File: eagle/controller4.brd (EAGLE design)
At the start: 117.8 x 48.2 mm, 30 parts, among them K1 SRD-05VDC-SL-C, K2 SRD-05VDC-SL-C, K3 SRD-05VDC-SL-C, K4 SRD-05VDC-SL-C, T1 BC547, T2 BC547, T3 BC547, T4 BC547, X1 VCC, X2 IN1, X3 IN2, X4 IN3, X5 IN4

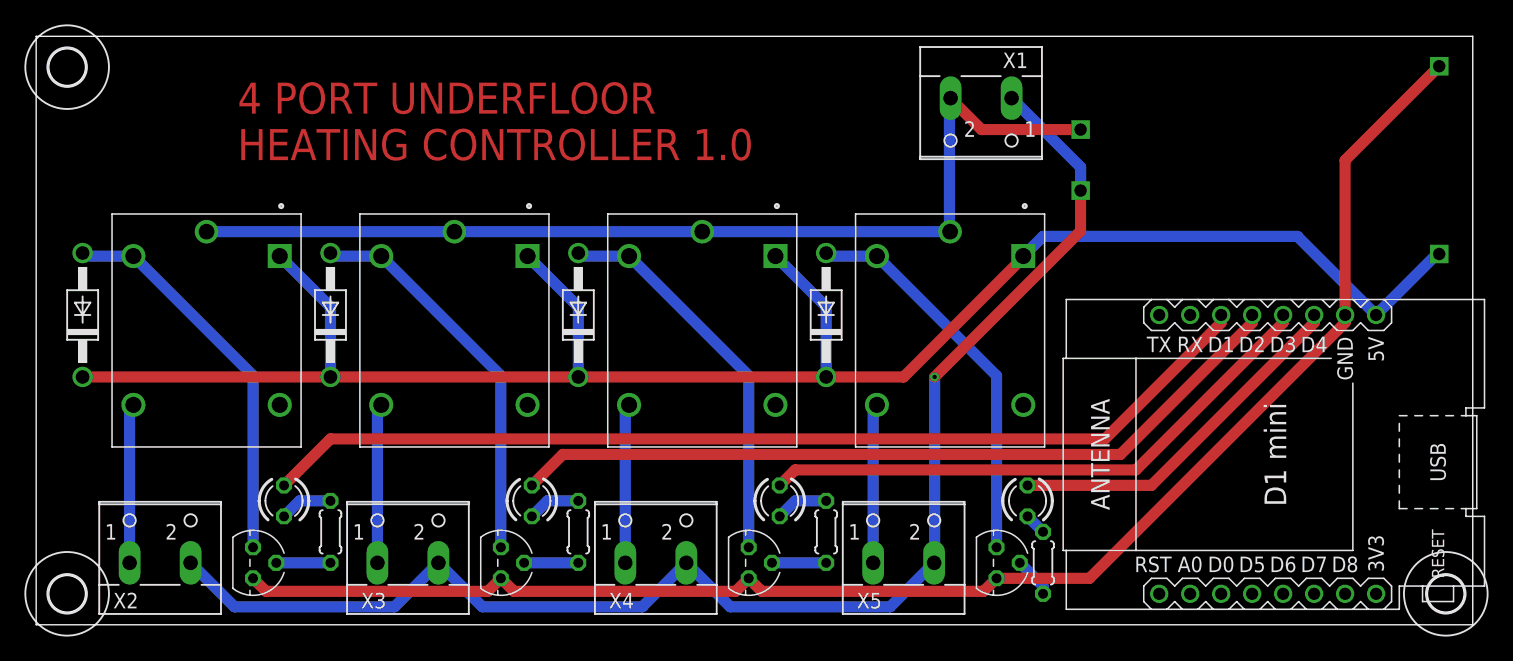
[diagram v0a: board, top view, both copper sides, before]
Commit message: Update to Version 1.1
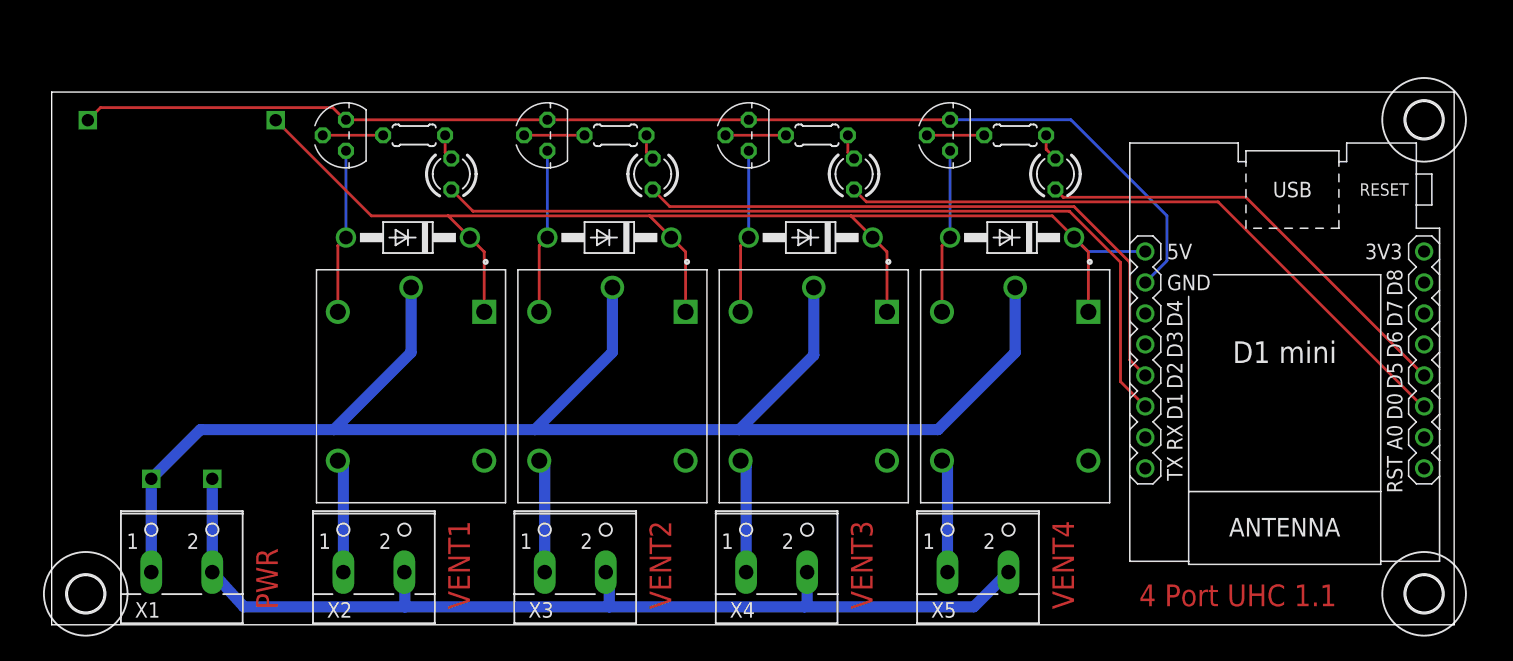
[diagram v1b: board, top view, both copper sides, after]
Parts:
- moved U$2 119.3 mm to (112.5, 2.54)
- moved HLK1 89.1 mm to (10.7, 26.7), turned to 90 degrees
- moved X1 74.9 mm to (10.7, 5.59), turned to 0 degrees
- moved U$4 38.9 mm to (112.5, 41.4)
- moved T1 35.9 mm to (24.1, 40.1), turned to 90 degrees
- moved T2 35.3 mm to (40.6, 40.1), turned to 90 degrees
- moved T4 35.3 mm to (73.7, 40.1), turned to 90 degrees
- moved R4 35.1 mm to (79.0, 40.1), turned to 180 degrees
- moved T3 35.1 mm to (57.1, 40.1), turned to 90 degrees
- moved R1 33.2 mm to (29.7, 40.1), turned to 180 degrees
- moved R2 32.7 mm to (46.2, 40.1), turned to 180 degrees
- moved R3 32.5 mm to (62.7, 40.1), turned to 180 degrees
- moved LED1 30.1 mm to (32.8, 37.0), turned to 90 degrees
- moved LED2 28.6 mm to (49.3, 37.0), turned to 90 degrees
- moved LED3 27.5 mm to (65.8, 37.0), turned to 90 degrees
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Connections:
- net 0V: now also X1.2; no longer X1.1
- net N$16: now also LED4.A, U$1.JP1.4; no longer LED3.A, U$1.JP2.5
- net N$17: now also LED3.A, U$1.JP1.3; no longer LED4.A, U$1.JP2.6
- net VCC: now also X1.1; no longer X1.2
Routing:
- net VCC: track 83.7 -> 130.8 mm
- net +5V: track 156.0 -> 109.6 mm
- net 0V: track 115.6 -> 84.3 mm, vias 1 -> 0
- net GND: track 125.1 -> 98.8 mm
- net N$17: track 29.7 -> 54.1 mm
- net N$4: track 32.2 -> 13.5 mm
- net N$3: track 32.2 -> 13.5 mm
- net N$5: track 32.2 -> 13.6 mm
- net N$1: track 32.2 -> 13.6 mm
- net N$14: track 65.2 -> 51.4 mm
- net N$15: track 83.0 -> 70.0 mm
- net N$16: track 47.4 -> 36.5 mm
- net N$13: track 13.1 -> 9.33 mm
- net N$12: track 13.1 -> 9.33 mm
- net N$2: track 13.1 -> 9.33 mm
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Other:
- board size 117.8 x 48.2 mm -> 115 x 43.7 mm
- board text added: "4 Port UHC 1.1"
- board text added: "PWR"
- board text added: "VENT1"
- board text added: "VENT2"
- board text added: "VENT3"
- board text added: "VENT4"
- board text removed: "4 PORT UNDERFLOOR HEATING CONTROLLER 1.0"
